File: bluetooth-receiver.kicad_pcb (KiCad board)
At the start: 2 copper layers, 45 x 33.6 mm, 11 parts, among them J1 Barrel_Jack_Switch, J3 RCJ-22, SW1 PAUSE, SW2 NEXT, SW3 PREV, SW4 ON_OFF, U1 m18, U2 dd1718pa

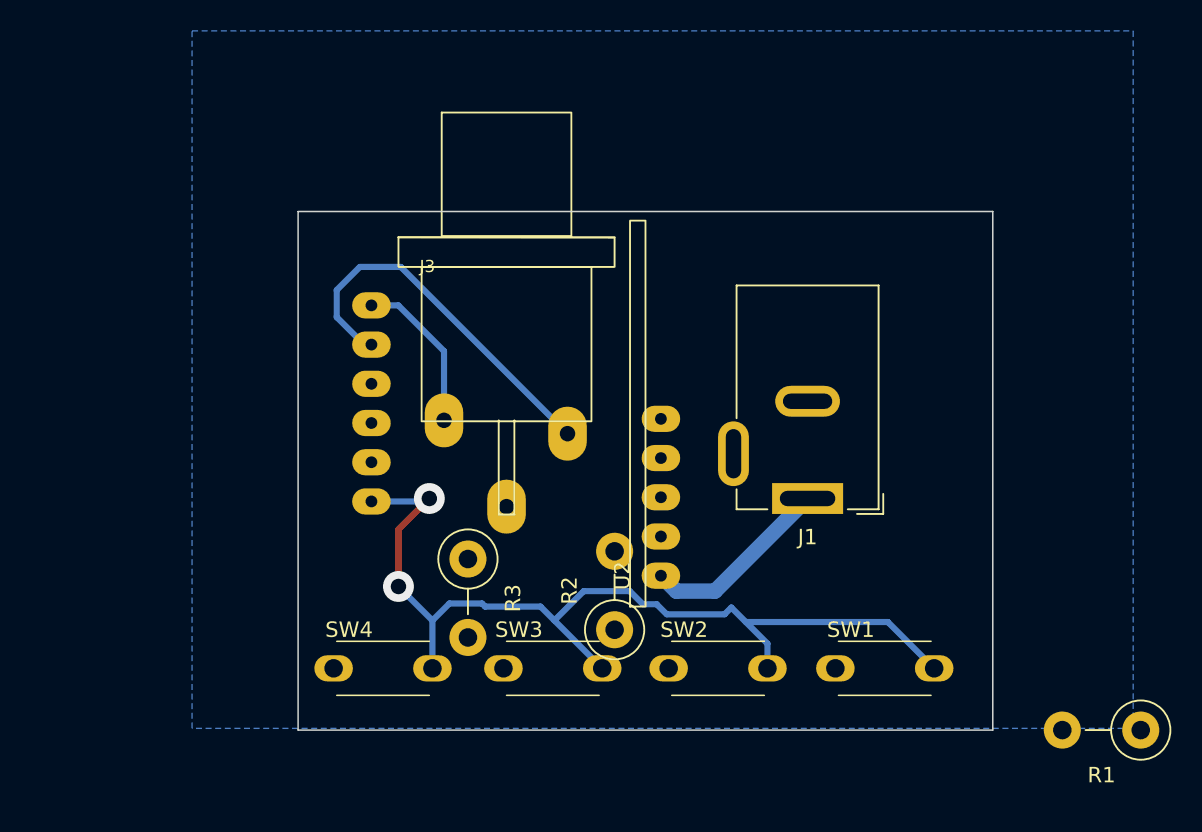
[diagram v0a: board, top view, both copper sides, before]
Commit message: Prepare for milling
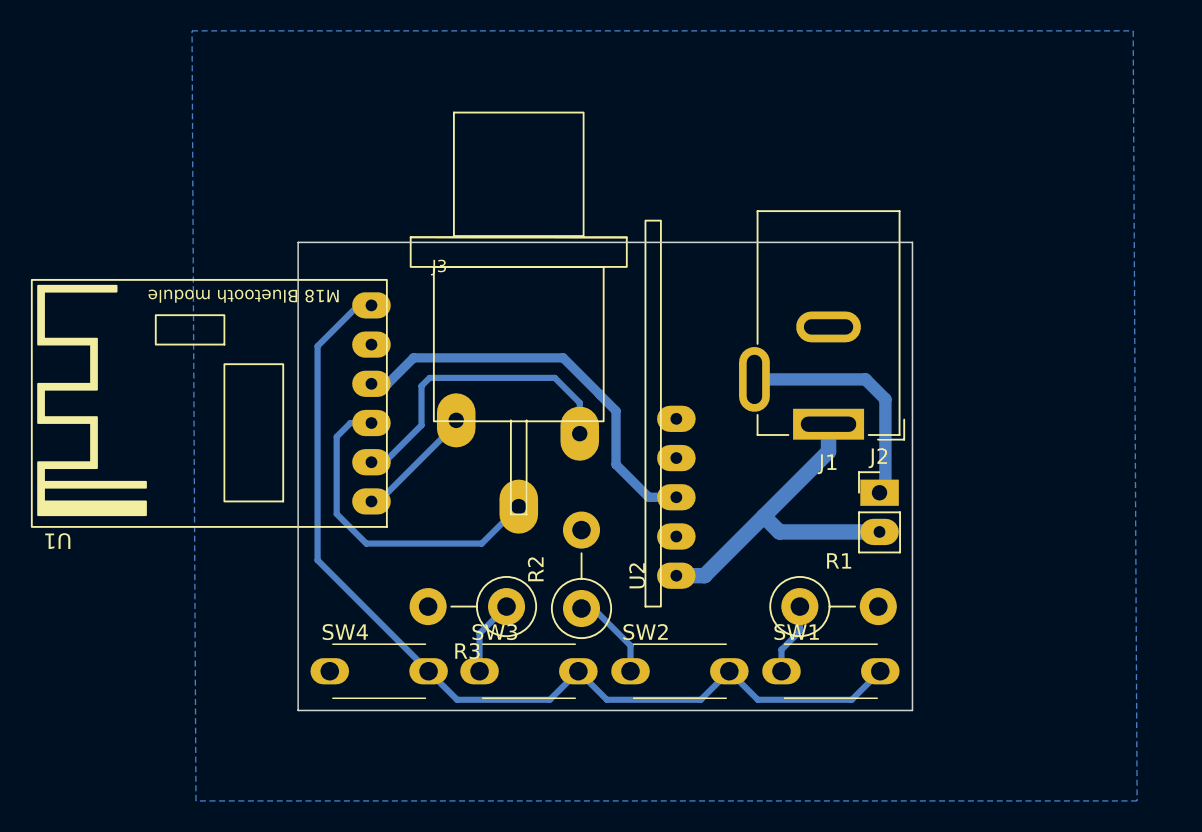
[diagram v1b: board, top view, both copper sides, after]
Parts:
- added J2: Power, Connector_PinHeader_2.54mm:PinHeader_1x02_P2.54mm_Vertical, F.Cu at (137.2, 95.6)
- U1: moved to F.Cu
- moved R1 23.5 mm to (132.0, 103.0), turned to 0 degrees
- moved J1 5.00 mm to (133.9, 91.2)
- moved R3 3.97 mm to (113.0, 103.0), turned to 180 degrees
- moved SW1 3.50 mm to (130.8, 107.2)
- moved R2 2.55 mm to (117.9, 103.1)
- moved SW2 2.48 mm to (121.0, 107.2)
- moved SW3 1.56 mm to (111.3, 107.2)
- moved U2 1.00 mm to (124.0, 101.0)
- moved J3 0.79 mm to (113.8, 91.0)
- moved SW4 0.31 mm to (101.5, 107.2)
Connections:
- J1 pad 3: unconnected-(J1-Pad3) -> Net-(J2-Pin_1)
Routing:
- net +5V: track 0.00 -> 26.2 mm
- net GND: track 0.00 -> 21.2 mm
- net Net-(J2-Pin_1): track 0.00 -> 15.2 mm
- net VBUS: track 12.4 -> 22.9 mm
- net Net-(R2-Pad1): track 0.00 -> 5.83 mm
- net Net-(R3-Pad1): track 0.00 -> 4.91 mm
- net /L: track 24.8 -> 19.9 mm
- net Net-(R1-Pad1): track 0.00 -> 4.68 mm
- net /R: track 10.4 -> 7.81 mm
- net Net-(U1-KEY): track 61.2 -> 62.5 mm, vias 2 -> 0
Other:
- board size 45 x 33.6 mm -> 39.8 x 30.3 mm
